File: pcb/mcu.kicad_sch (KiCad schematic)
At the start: 29 parts, among them J201 eflashy32, J203 Input, SW201 RESET, U201 ESP32-S3R8, U202 W25Q128JVSIQ, Y201 40MHz

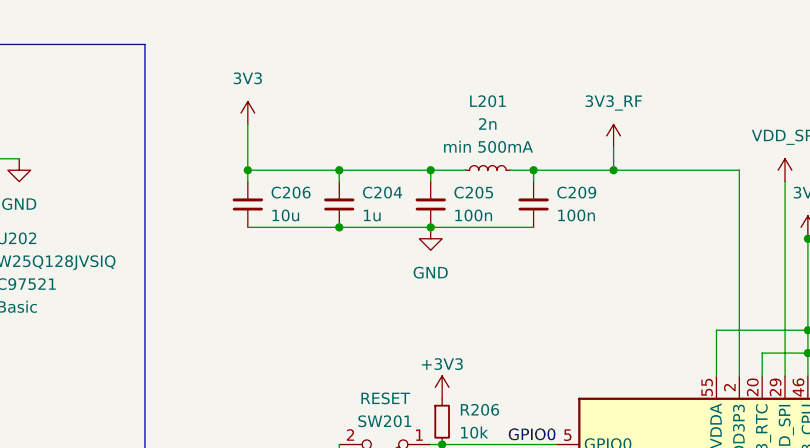
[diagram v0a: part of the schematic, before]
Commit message: schematic and tweaks
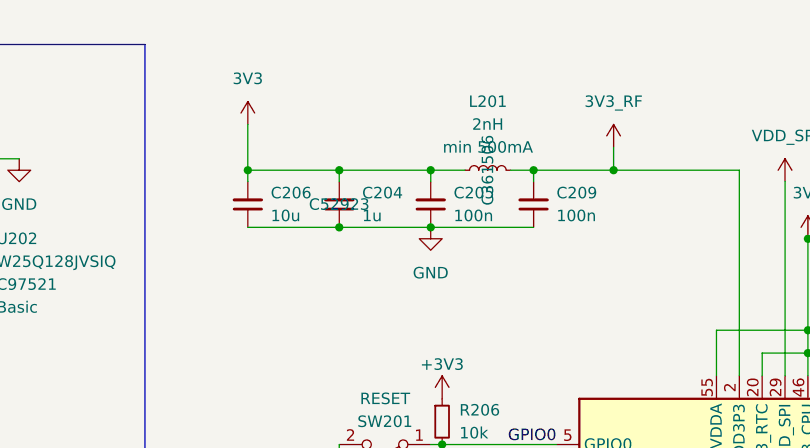
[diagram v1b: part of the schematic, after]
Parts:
- C203, C205, C207, C209, C212, C213, C214: footprint (none) -> Capacitor_SMD:C_0402_1005Metric; LCSC (none) -> C307331
- C204: footprint (none) -> Capacitor_SMD:C_0402_1005Metric; LCSC (none) -> C52923
- C206: footprint (none) -> Capacitor_SMD:C_0603_1608Metric; LCSC (none) -> C96446
- C208: footprint Capacitor_SMD:C_0805_2012Metric -> Capacitor_SMD:C_0603_1608Metric; LCSC C15850 -> C96446
- J203: LCSC (none) -> C3168400
- L201: value 2n -> 2nH; footprint (none) -> Inductor_SMD:L_0402_1005Metric; LCSC (none) -> C361506
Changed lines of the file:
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@@
 			)
 		)
-		(property "Footprint" ""
+		(property "Footprint" "Capacitor_SMD:C_0402_1005Metric"
 			(at 177.8 43.18 0)
 			(effects
@@
 			)
 		)
+		(property "LCSC" "C307331"
+			(at 177.8 43.18 0)
+			(effects
+				(font
+					(size 1.27 1.27)
+				)
+				(hide yes)
+			)
+		)
 		(pin "1"
 		)
@@
 			)
 		)
+		(property "LCSC" "C3168400"
+			(at 241.3 74.93 0)
+			(effects
+				(font
+					(size 1.27 1.27)
+				)
+				(hide yes)
+			)
+		)
 		(pin "7"
 		)
@@
 			)
 		)
-		(property "Footprint" ""
+		(property "Footprint" "Capacitor_SMD:C_0402_1005Metric"
 			(at 46.99 31.75 0)
 			(effects
@@
 			)
 		)
+		(property "LCSC" "C307331"
+			(at 46.99 31.75 0)
+			(effects
+				(font
+					(size 1.27 1.27)
+				)
+				(hide yes)
+			)
+		)
 		(pin "1"
 		)
@@
 			)
 		)
-		(property "Footprint" "Capacitor_SMD:C_0805_2012Metric"
+		(property "Footprint" "Capacitor_SMD:C_0603_1608Metric"
 			(at 175.26 130.81 0)
 			(effects
@@
 			)
 		)
-		(property "LCSC" "C15850"
+		(property "LCSC" "C96446"
 			(at 175.26 130.81 0)
 			(effects
@@
 			)
 		)
-		(property "Footprint" ""
+		(property "Footprint" "Capacitor_SMD:C_0402_1005Metric"
 			(at 167.64 43.18 0)
 			(effects
@@
 			)
 		)
+		(property "LCSC" "C307331"
+			(at 167.64 43.18 0)
+			(effects
+				(font
+					(size 1.27 1.27)
+				)
+				(hide yes)
+			)
+		)
 		(pin "1"
 		)
@@
 			)
 		)
-		(property "Value" "2n"
+		(property "Value" "2nH"
 			(at 105.41 27.94 90)
 			(effects
@@
 			)
 		)
-		(property "Footprint" ""
+		(property "Footprint" "Inductor_SMD:L_0402_1005Metric"
 			(at 105.41 33.02 0)
 			(effects
@@
 			)
 		)
-		(property "LCSC" ""
+		(property "LCSC" "C361506"
 			(at 105.41 33.02 0)
 			(effects
@@
 			)
 		)
-		(property "Footprint" ""
+		(property "Footprint" "Capacitor_SMD:C_0402_1005Metric"
 			(at 99.06 36.83 0)
 			(effects
@@
 			)
 		)
+		(property "LCSC" "C307331"
+			(at 99.06 36.83 0)
+			(effects
+				(font
+					(size 1.27 1.27)
+				)
+				(hide yes)
+			)
+		)
 		(pin "1"
 		)
@@
 			)
 		)
-		(property "Footprint" ""
+		(property "Footprint" "Capacitor_SMD:C_0402_1005Metric"
 			(at 110.49 36.83 0)
 			(effects
@@
 			)
 		)
+		(property "LCSC" "C307331"
+			(at 110.49 36.83 0)
+			(effects
+				(font
+					(size 1.27 1.27)
+				)
+				(hide yes)
+			)
+		)
 		(pin "1"
 		)
@@
 			)
 		)
-		(property "Footprint" ""
+		(property "Footprint" "Capacitor_SMD:C_0402_1005Metric"
 			(at 88.9 36.83 0)
 			(effects
@@
 			)
 		)
-		(property "LCSC" ""
+		(property "LCSC" "C52923"
 			(at 88.9 36.83 0)
 			(effects
@@
 			)
 		)
-		(property "Footprint" ""
+		(property "Footprint" "Capacitor_SMD:C_0603_1608Metric"
 			(at 78.74 36.83 0)
 			(effects
@@
 			)
 		)
+		(property "LCSC" "C96446"
+			(at 78.74 36.83 0)
+			(effects
+				(font
+					(size 1.27 1.27)
+				)
+				(hide yes)
+			)
+		)
+		(property "Notes" ""
+			(at 78.74 36.83 0)
+			(effects
+				(font
+					(size 1.27 1.27)
+				)
+			)
+		)
 		(pin "1"
 		)
@@
 			)
 		)
-		(property "Footprint" ""
+		(property "Footprint" "Capacitor_SMD:C_0402_1005Metric"
 			(at 146.05 43.18 0)
 			(effects
@@
 			)
 		)
+		(property "LCSC" "C307331"
+			(at 146.05 43.18 0)
+			(effects
+				(font
+					(size 1.27 1.27)
+				)
+				(hide yes)
+			)
+		)
 		(pin "1"
 		)
@@
 			)
 		)
-		(property "Footprint" ""
+		(property "Footprint" "Capacitor_SMD:C_0402_1005Metric"
 			(at 157.48 43.18 0)
 			(effects
@@
 			(at 157.48 43.18 0)
 			(effects
+				(font
+					(size 1.27 1.27)
+				)
+				(hide yes)
+			)
+		)
+		(property "LCSC" "C307331"
+			(at 157.48 43.18 0)
+			(effects

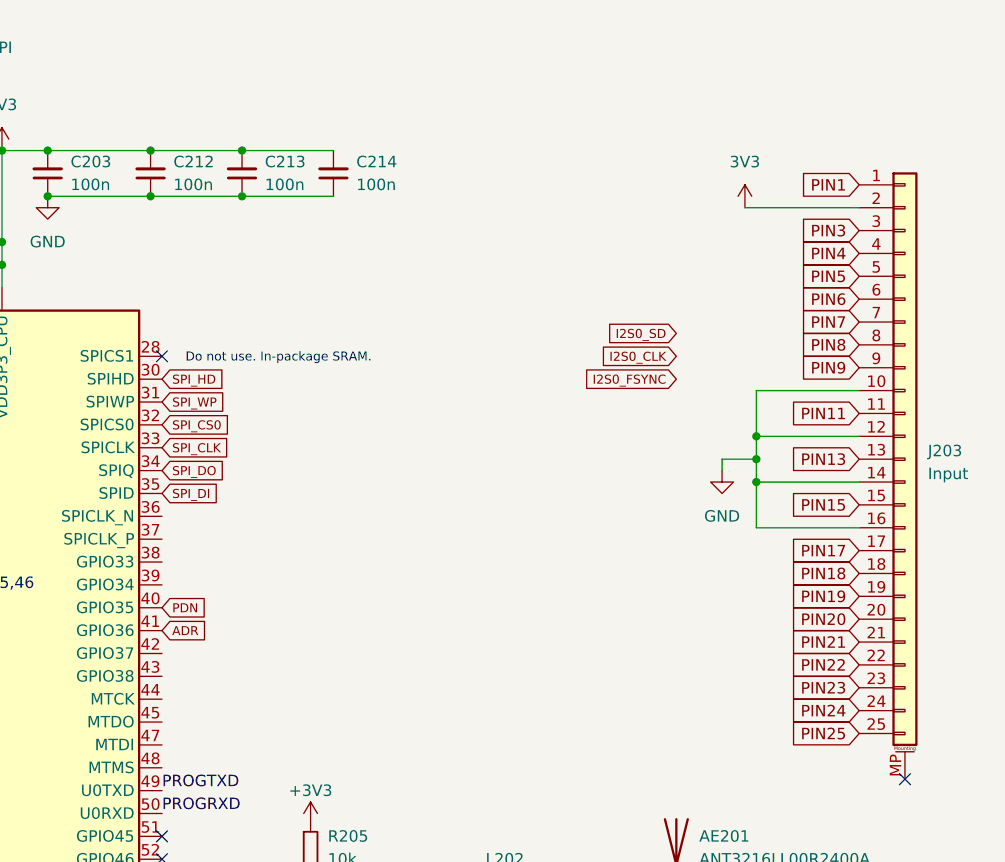
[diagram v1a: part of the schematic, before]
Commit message: up
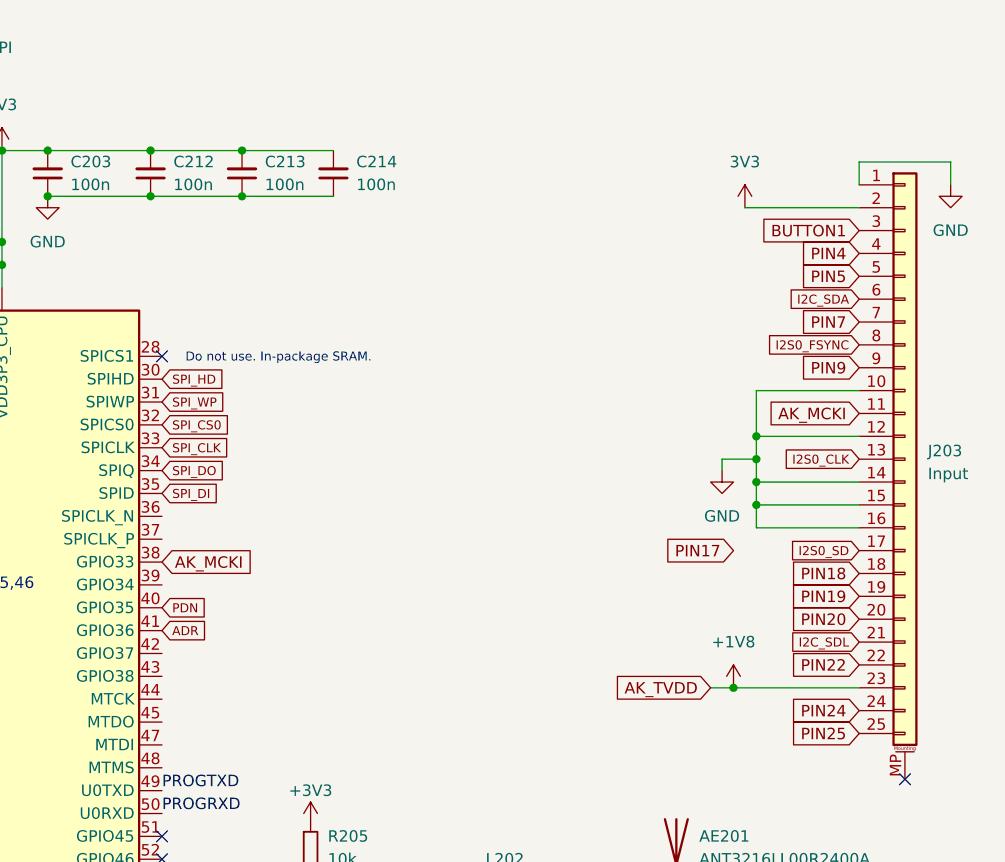
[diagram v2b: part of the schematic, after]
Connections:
- net PIN1 is gone; now on net GND: J203.1 (Pin_1)
- net PIN11 is gone; now on net AK_MCKI: J203.11 (Pin_11)
- net PIN13 is gone; now on net I2S0_CLK: J203.13 (Pin_13)
- net PIN15 is gone; now on net GND: J203.15 (Pin_15)
- net PIN21 is gone; now on net I2C_SDL: J203.21 (Pin_21)
- net PIN6 is gone; now on net I2C_SDA: J203.6 (Pin_6)
- net PIN8 is gone; now on net I2S0_FSYNC: J203.8 (Pin_8)
- net I2S0_SD: now also J203.17 (Pin_17)
- net PIN17: no longer J203.17 (Pin_17)
- net AK_MCKI: now reaches U201.38 (GPIO33)
- net PIN23 renamed +1V8
- net PIN3 renamed BUTTON1
